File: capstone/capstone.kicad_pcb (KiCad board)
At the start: 2 copper layers, 77.9 x 74.8 mm, 15 parts, among them J1 Conn_01x02, M1 Motor_Servo, M2 Motor_Servo, M3 Stepper_Motor_bipolar, M4 Stepper_Motor_bipolar, SW1 SW_Push, U1 PicoW

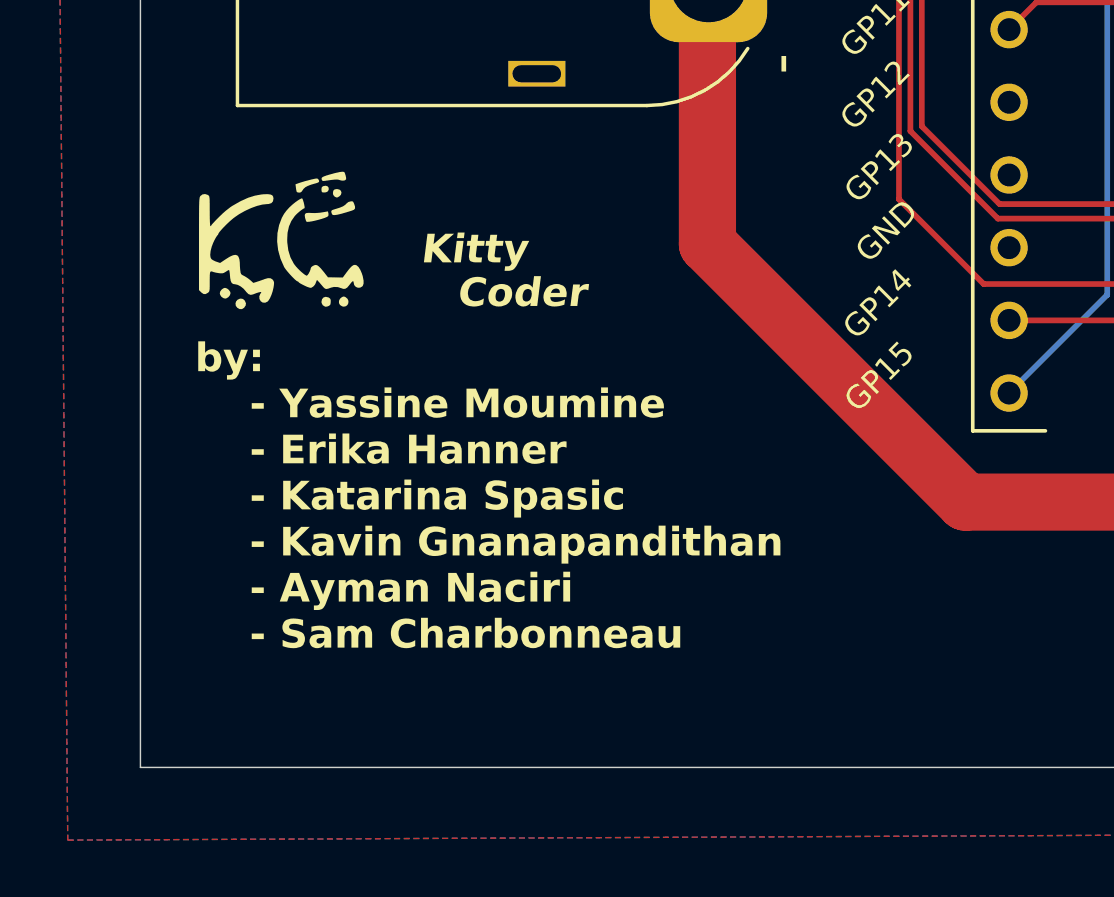
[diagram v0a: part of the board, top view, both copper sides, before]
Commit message: text design
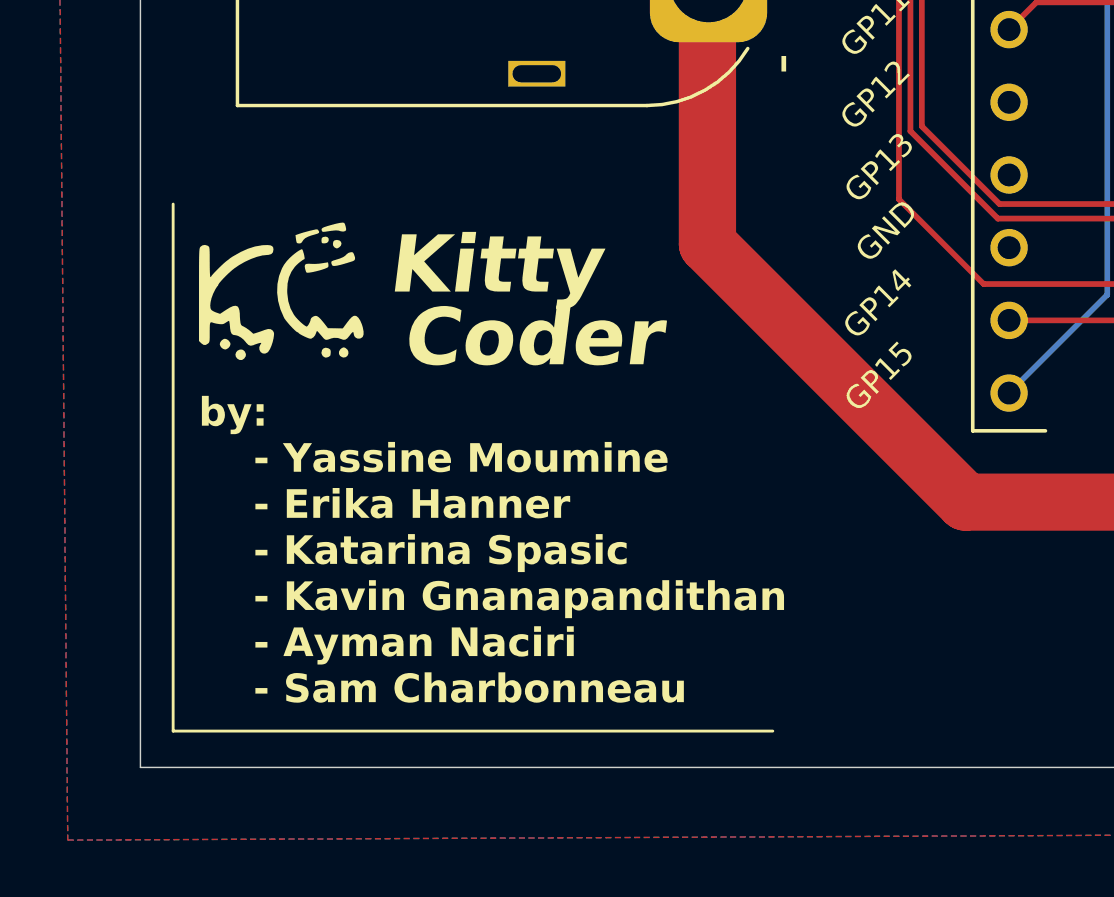
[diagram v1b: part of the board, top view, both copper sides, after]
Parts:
- moved G*** 1.78 mm to (62.1, 144.3)
